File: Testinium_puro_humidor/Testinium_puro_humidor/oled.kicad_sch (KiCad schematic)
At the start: 0 parts

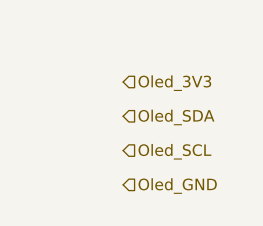
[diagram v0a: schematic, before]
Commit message: sematik tamamlandi
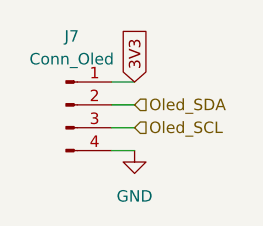
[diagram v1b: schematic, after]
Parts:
- added J7: Conn_Oled, Connector_JST:JST_EH_B4B-EH-A_1x04_P2.50mm_Vertical, symbol Connector:Conn_01x04_Pin
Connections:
- net Oled_SCL: now also J7.3 (Pin_3)
- net Oled_SDA: now also J7.2 (Pin_2)
- new net 3V3: J7.1 (Pin_1)
- new net GND: J7.4 (Pin_4)
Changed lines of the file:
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@@
 	(generator_version "9.0")
 	(paper "A4")
-	(hierarchical_label "Oled_SCL"
+	(wire
+		(pts
+			(xy 25.4 31.75) (xy 22.86 31.75)
+		)
+		(stroke
+			(width 0)
+			(type default)
+		)
+	)
+	(wire
+		(pts
+			(xy 25.4 36.83) (xy 22.86 36.83)
+		)
+		(stroke
+			(width 0)
+			(type default)
+		)
+	)
+	(wire
+		(pts
+			(xy 25.4 29.21) (xy 22.86 29.21)
+		)
+		(stroke
+			(width 0)
+			(type default)
+		)
+	)
+	(wire
+		(pts
+			(xy 25.4 34.29) (xy 22.86 34.29)
+		)
+		(stroke
+			(width 0)
+			(type default)
+		)
+	)
+	(global_label "3V3"
 		(shape input)
-		(at 24.13 36.83 0)
+		(at 25.4 29.21 90)
+		(fields_autoplaced yes)
 		(effects
 			(font
@@
 			(justify left)
 		)
-	)
-	(hierarchical_label "Oled_GND"
+		(property "Intersheetrefs" "${INTERSHEET_REFS}"
+			(at 25.4 22.7172 90)
+			(effects
+				(font
+					(size 1.27 1.27)
+				)
+				(justify left)
+				(hide yes)
+			)
+		)
+	)
+	(hierarchical_label "Oled_SCL"
 		(shape input)
-		(at 24.13 40.64 0)
+		(at 25.4 34.29 0)
 		(effects
 			(font
@@
 		)
 	)
-	(hierarchical_label "Oled_3V3"
+	(hierarchical_label "Oled_SDA"
 		(shape input)
-		(at 24.13 29.21 0)
+		(at 25.4 31.75 0)
 		(effects
 			(font
@@
 		)
 	)
-	(hierarchical_label "Oled_SDA"
-		(shape input)
-		(at 24.13 33.02 0)
-		(effects
-			(font
-				(size 1.27 1.27)
-			)
-			(justify left)
-		)
-	)
+	(symbol
+		(lib_id "Connector:Conn_01x04_Pin")
+		(at 17.78 31.75 0)
+		(unit 1)
+		(exclude_from_sim no)
+		(in_bom yes)
+		(on_board yes)
+		(dnp no)
+		(fields_autoplaced yes)
+		(property "Reference" "J7"
+			(at 18.415 24.13 0)
+			(effects
+				(font
+					(size 1.27 1.27)
+				)
+			)
+		)
+		(property "Value" "Conn_Oled"
+			(at 18.415 26.67 0)
+			(effects
+				(font
+					(size 1.27 1.27)
+				)
+			)
+		)
+		(property "Footprint" "Connector_JST:JST_EH_B4B-EH-A_1x04_P2.50mm_Vertical"
+			(at 17.78 31.75 0)
+			(effects
+				(font
+					(size 1.27 1.27)
+				)
+				(hide yes)
+			)
+		)
+		(property "Datasheet" "~"
+			(at 17.78 31.75 0)
+			(effects
+				(font
+					(size 1.27 1.27)
+				)
+				(hide yes)
+			)
+		)
+		(property "Description" "Generic connector, single row, 01x04, script generated"
+			(at 17.78 31.75 0)
+			(effects
+				(font
+					(size 1.27 1.27)
+				)
+				(hide yes)
+			)
+		)
+		(pin "4"
+		)
+		(pin "1"
+		)
+		(pin "2"
+		)
+		(pin "3"
+		)
+		(instances
+			(project "Testinium_puro_humidor"
+				(path "/eaf24445-473d-4e1b-a90d-ef2c4a02e74f/de88d65f-a1ab-4785-a813-62ea466efae0"
+					(reference "J7")
+					(unit 1)
+				)
+			)
+		)
+	)
+	(symbol
+		(lib_id "power:GND")
+		(at 25.4 36.83 0)
+		(unit 1)
+		(exclude_from_sim no)
+		(in_bom yes)
+		(on_board yes)
+		(dnp no)
+		(fields_autoplaced yes)
+		(property "Reference" "#PWR09"
+			(at 25.4 43.18 0)
+			(effects
+				(font
+					(size 1.27 1.27)
+				)
+				(hide yes)
+			)
+		)
+		(property "Value" "GND"
+			(at 25.4 41.91 0)
+			(effects
+				(font
+					(size 1.27 1.27)
+				)
+			)
+		)
+		(property "Footprint" ""
+			(at 25.4 36.83 0)
+			(effects
+				(font
+					(size 1.27 1.27)
+				)
+				(hide yes)
+			)
+		)
+		(property "Datasheet" ""
+			(at 25.4 36.83 0)
+			(effects
+				(font
+					(size 1.27 1.27)
+				)
+				(hide yes)
+			)
+		)
+		(property "Description" "Power symbol creates a global label with name \"GND\" , ground"
+			(at 25.4 36.83 0)
+			(effects
+				(font
+					(size 1.27 1.27)
+				)
+				(hide yes)
+			)
+		)
+		(pin "1"
+		)
+		(instances
+			(project "Testinium_puro_humidor"
+				(path "/eaf24445-473d-4e1b-a90d-ef2c4a02e74f/de88d65f-a1ab-4785-a813-62ea466efae0"
+					(reference "#PWR09")
+					(unit 1)
+				)
+			)
+		)
+	)
